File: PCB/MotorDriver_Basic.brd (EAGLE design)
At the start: 27.1 x 36.8 mm, 17 parts, among them IC1 MPU6050, U1 DRV8835

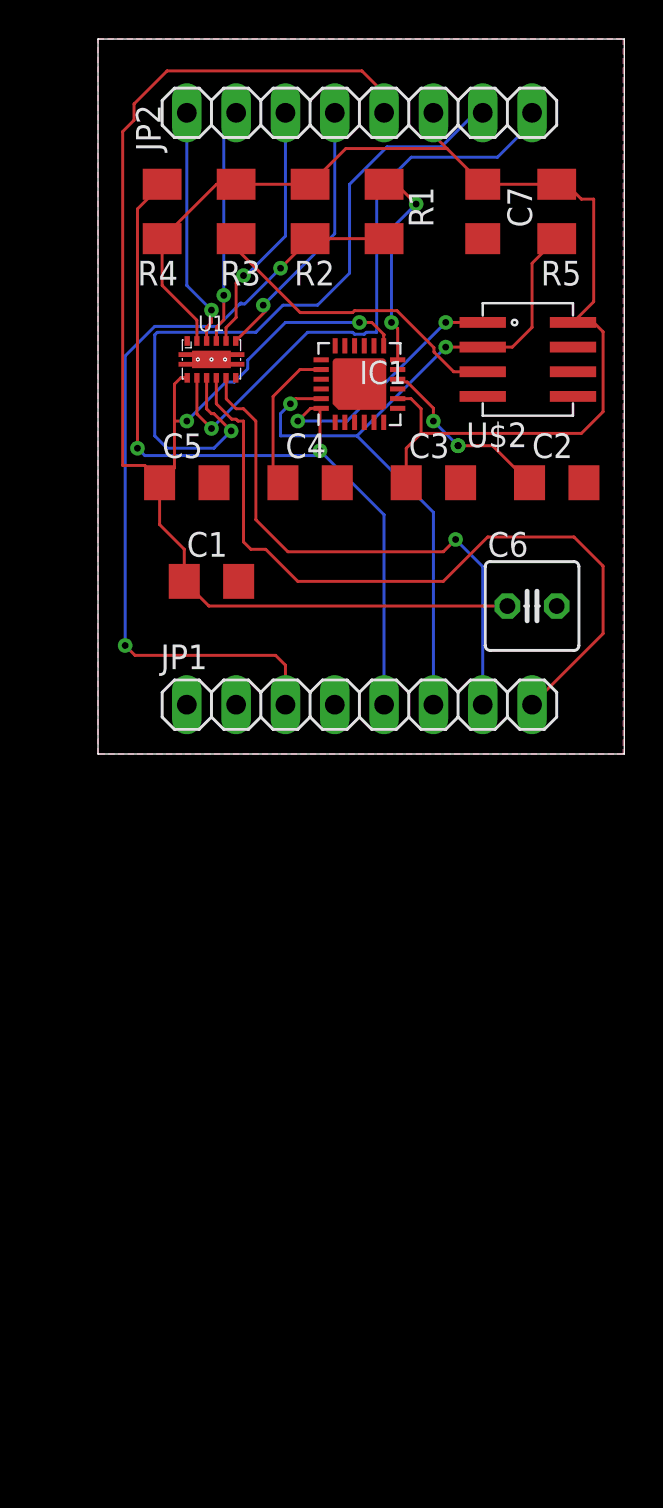
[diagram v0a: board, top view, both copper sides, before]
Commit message: Tweaked the board file
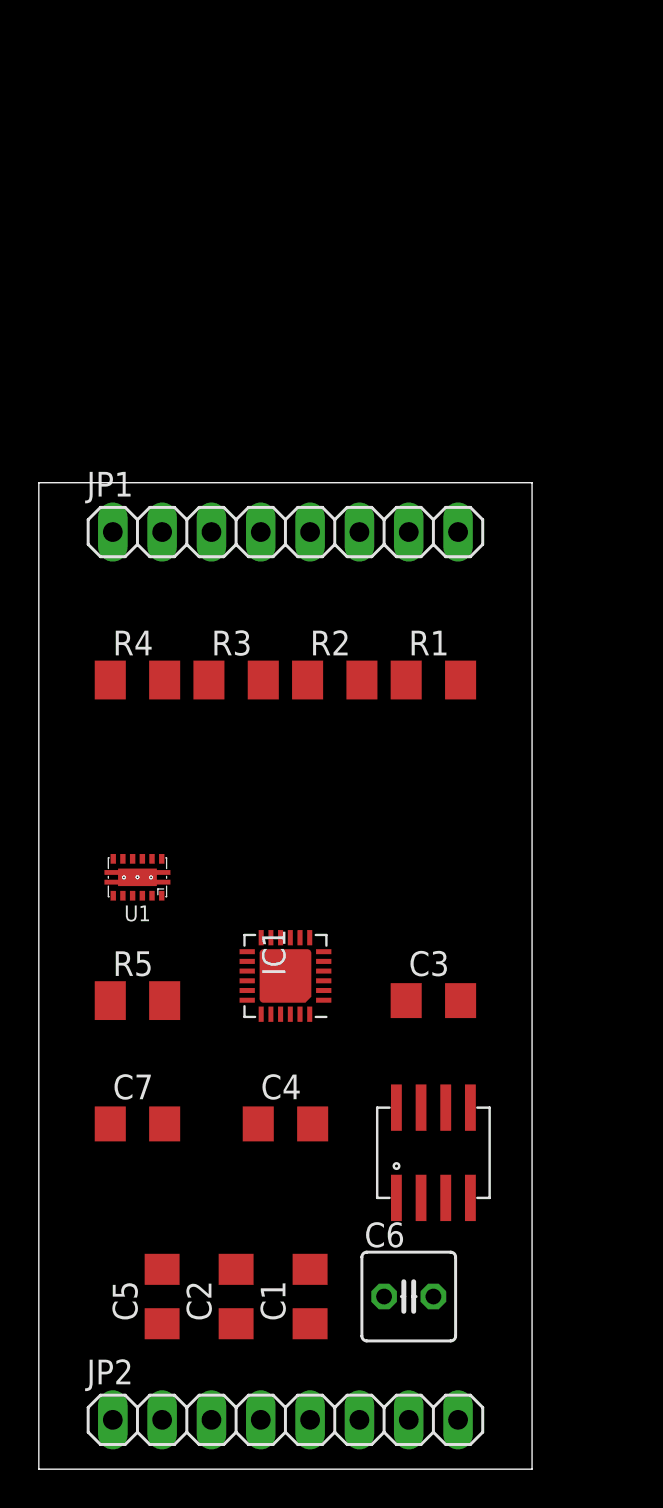
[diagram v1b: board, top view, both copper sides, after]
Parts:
- moved JP2 67.4 mm to (12.7, 2.54)
- moved C7 50.2 mm to (5.08, 17.8), turned to 0 degrees
- moved R5 46.0 mm to (5.08, 24.1), turned to 0 degrees
- moved C2 45.0 mm to (10.2, 8.89), turned to 90 degrees
- moved C5 41.9 mm to (6.35, 8.89), turned to 90 degrees
- moved U$2 41.0 mm to (20.3, 16.5), turned to 90 degrees
- moved C1 37.2 mm to (14.0, 8.89), turned to 90 degrees
- moved C6 36.1 mm to (19.1, 8.89)
- moved C4 33.0 mm to (12.7, 17.8)
- moved IC1 30.7 mm to (12.7, 25.4), turned to 90 degrees
- moved U1 26.9 mm to (5.08, 30.5), turned to 180 degrees
- moved C3 26.7 mm to (20.3, 24.1)
- moved R1 24.3 mm to (20.3, 40.6), turned to 0 degrees
- moved R2 24.2 mm to (15.2, 40.6), turned to 0 degrees
- moved R4 24.2 mm to (5.08, 40.6), turned to 0 degrees
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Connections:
- net AIN1: now also JP2.4; no longer JP2.1
- net AIN2: now also JP2.3; no longer JP2.2
- net BIN1: now also JP2.2; no longer JP2.3
- net BIN2: now also JP2.1; no longer JP2.4
- net GND: now also JP1.5, JP2.5, JP2.6; no longer JP1.1, JP1.2, JP1.4
- net IMU_INT: now also JP1.8; no longer JP1.3
- net MOUTA1: now also JP1.4; no longer JP2.8
- net MOUTA2: now also JP1.3; no longer JP2.7
- net MOUTB1: now also JP1.2; no longer JP1.8
- net MOUTB2: now also JP1.1; no longer JP1.7
- net SCL: now also JP2.7; no longer JP1.6
- net SDA: now also JP2.8; no longer JP1.5
- net VCC: now also JP1.7; no longer JP2.6
- net VM: now also JP1.6; no longer JP2.5
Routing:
- net VM: track 79.2 -> 0.00 mm, vias 2 -> 0
- net VCC: track 62.2 -> 0.00 mm
- net SDA: track 53.5 -> 0.00 mm, vias 4 -> 0
- net IMU_INT: track 41.5 -> 0.00 mm, vias 2 -> 0
- net SCL: track 39.4 -> 0.00 mm, vias 2 -> 0
- net MOUTB1: track 38.9 -> 0.00 mm
- net MOUTA2: track 37.4 -> 0.00 mm, vias 1 -> 0
- net MOUTA1: track 30.8 -> 0.00 mm, vias 1 -> 0
- net MOUTB2: track 28.5 -> 0.00 mm, vias 1 -> 0
- net O.S.: track 16.0 -> 0.00 mm
- net BIN2: track 14.0 -> 0.00 mm, vias 1 -> 0
- net BIN1: track 13.1 -> 0.00 mm, vias 1 -> 0
- net AIN1: track 12.4 -> 0.00 mm, vias 1 -> 0
- net AIN2: track 12.2 -> 0.00 mm, vias 1 -> 0
- net N$2: track 10.8 -> 0.00 mm, vias 2 -> 0
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- removed copper zone on layer 1, net GND
- removed copper zone on layer 16, net GND
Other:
- board size 27.1 x 36.8 mm -> 25.4 x 50.8 mm
